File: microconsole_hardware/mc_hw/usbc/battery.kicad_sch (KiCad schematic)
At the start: 19 parts, among them J2 USB_C_Receptacle_USB2.0_16P, U23 S2B-PH-K-S, U24 S2B-PH-K-S, U6 MCP73833_MSOP

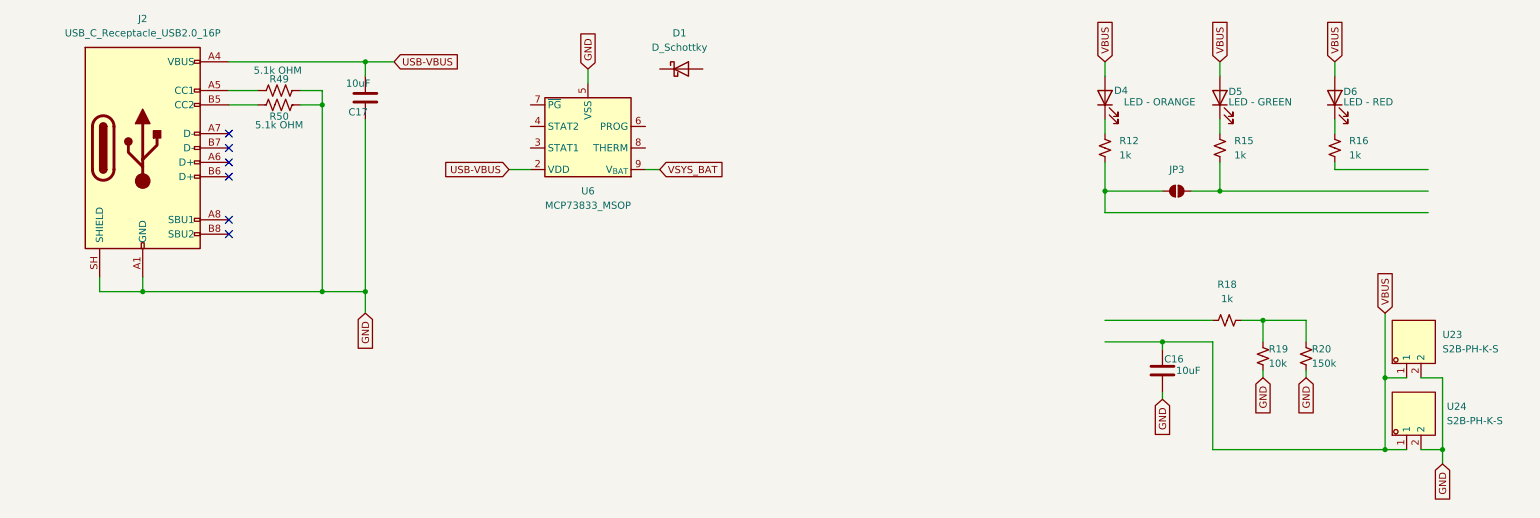
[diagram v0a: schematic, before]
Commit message: charging pass
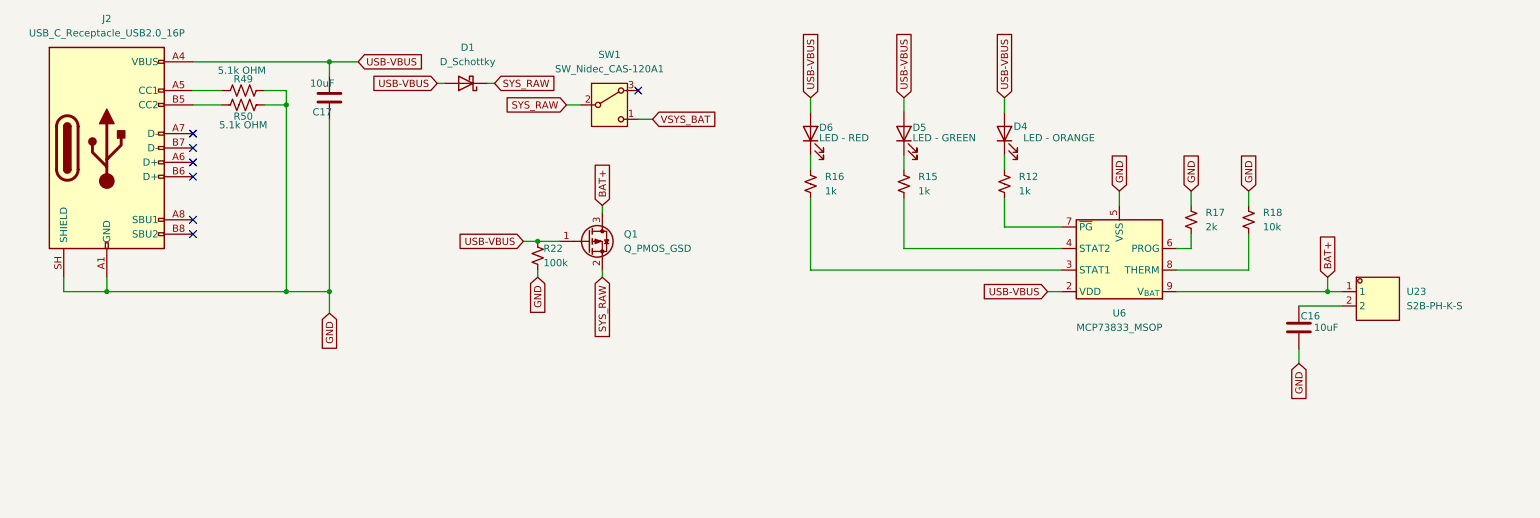
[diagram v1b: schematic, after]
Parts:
- removed JP3: (no value), PCM_SparkFun-Jumper:Jumper_2_NO, symbol PCM_SparkFun-Jumper:SolderJumper_2_Open
- removed R19: 10k, PCM_SparkFun-Resistor:R_0603_1608Metric, symbol PCM_SparkFun-Resistor:0.47_0603
- removed R20: 150k, PCM_SparkFun-Resistor:R_0603_1608Metric, symbol PCM_SparkFun-Resistor:0.47_0603
- removed U24: S2B-PH-K-S, project_parts:CONN-TH_S2B-PH-K-S-LF-SN, symbol project_parts:S2B-PH-K-S
- added Q1: Q_PMOS_GSD, symbol Transistor_FET:Q_PMOS_GSD
- added R17: 2k, PCM_SparkFun-Resistor:R_0603_1608Metric, symbol PCM_SparkFun-Resistor:0.47_0603
- added R22: 100k, PCM_SparkFun-Resistor:R_0603_1608Metric, symbol PCM_SparkFun-Resistor:0.47_0603
- added SW1: SW_Nidec_CAS-120A1, Button_Switch_SMD:Nidec_Copal_CAS-120A, symbol Switch:SW_Nidec_CAS-120A1
- R18: value 1k -> 10k
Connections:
- net GND: now also C16.2, R18.2, R17.2, R22.2; no longer C16.1, U23.2
- net VDD: now also D1.2 (A), D4.2 (A), D5.2 (A), D6.2 (A), Q1.1 (G), R22.1
- net VSYS_BAT: now also SW1.1 (C); no longer U6.10 (V_{BAT}), U6.9 (V_{BAT})
- net at R16.1: now also U6.3 (STAT1)
- net at R12.1: now also U6.7 (~{PG})
- net at R15.1: now also U6.4 (STAT2)
- net at U6.6 (PROG): now also R17.1
- net at U6.8 (THERM): now also R18.1
- net SYS_RAW: now reaches D1.1 (K)
- net SYS_RAW: now also Q1.2 (S), SW1.2 (B)
- removed net VBUS: C16.2, D4.2 (A), D5.2 (A), D6.2 (A), U23.1
- new net: C16.1, U23.2
- new net BAT+: Q1.3 (D), U23.1, U6.10 (V_{BAT}), U6.9 (V_{BAT})
- no-connect marks 6 -> 7
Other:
- moved on the sheet: C17, D6, J2, R16, R49, R50, U6

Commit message: PCB First Pass
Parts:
- J2: footprint (none) -> Connector_USB:USB_C_Receptacle_GCT_USB4135-GF-A_6P_TopMnt_Horizontal
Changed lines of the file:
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@@
 			)
 		)
-		(property "Footprint" ""
+		(property "Footprint" "Connector_USB:USB_C_Receptacle_GCT_USB4135-GF-A_6P_TopMnt_Horizontal"
 			(at 36.83 46.99 0)
 			(hide yes)
